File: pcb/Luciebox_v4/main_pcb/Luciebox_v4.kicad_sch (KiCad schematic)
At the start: 67 parts, among them J1 USB_B_Mini, P1 Power, P2 Analog, P3 Digital, P4 Digital, P5 CONN_01X01, P6 CONN_01X01, P7 CONN_01X01, P8 CONN_01X01, Q1 N-Channel_Mosfet, T1 terminal_3x1, T10 terminal_8x1, T11 terminal_8x1, T12 terminal_8x1, T13 terminal_8x1, T2 terminal_3x1, T3 terminal_3x1, T4 terminal_3x1, T5 terminal_8x1, T6 terminal_8x1, T7 terminal_3x1, T8 terminal_3x1, T9 terminal_3x1, U1 CA56-12SRWA, U2 8X8PADS, U3 ATmega328-PU, Y1 16MHz

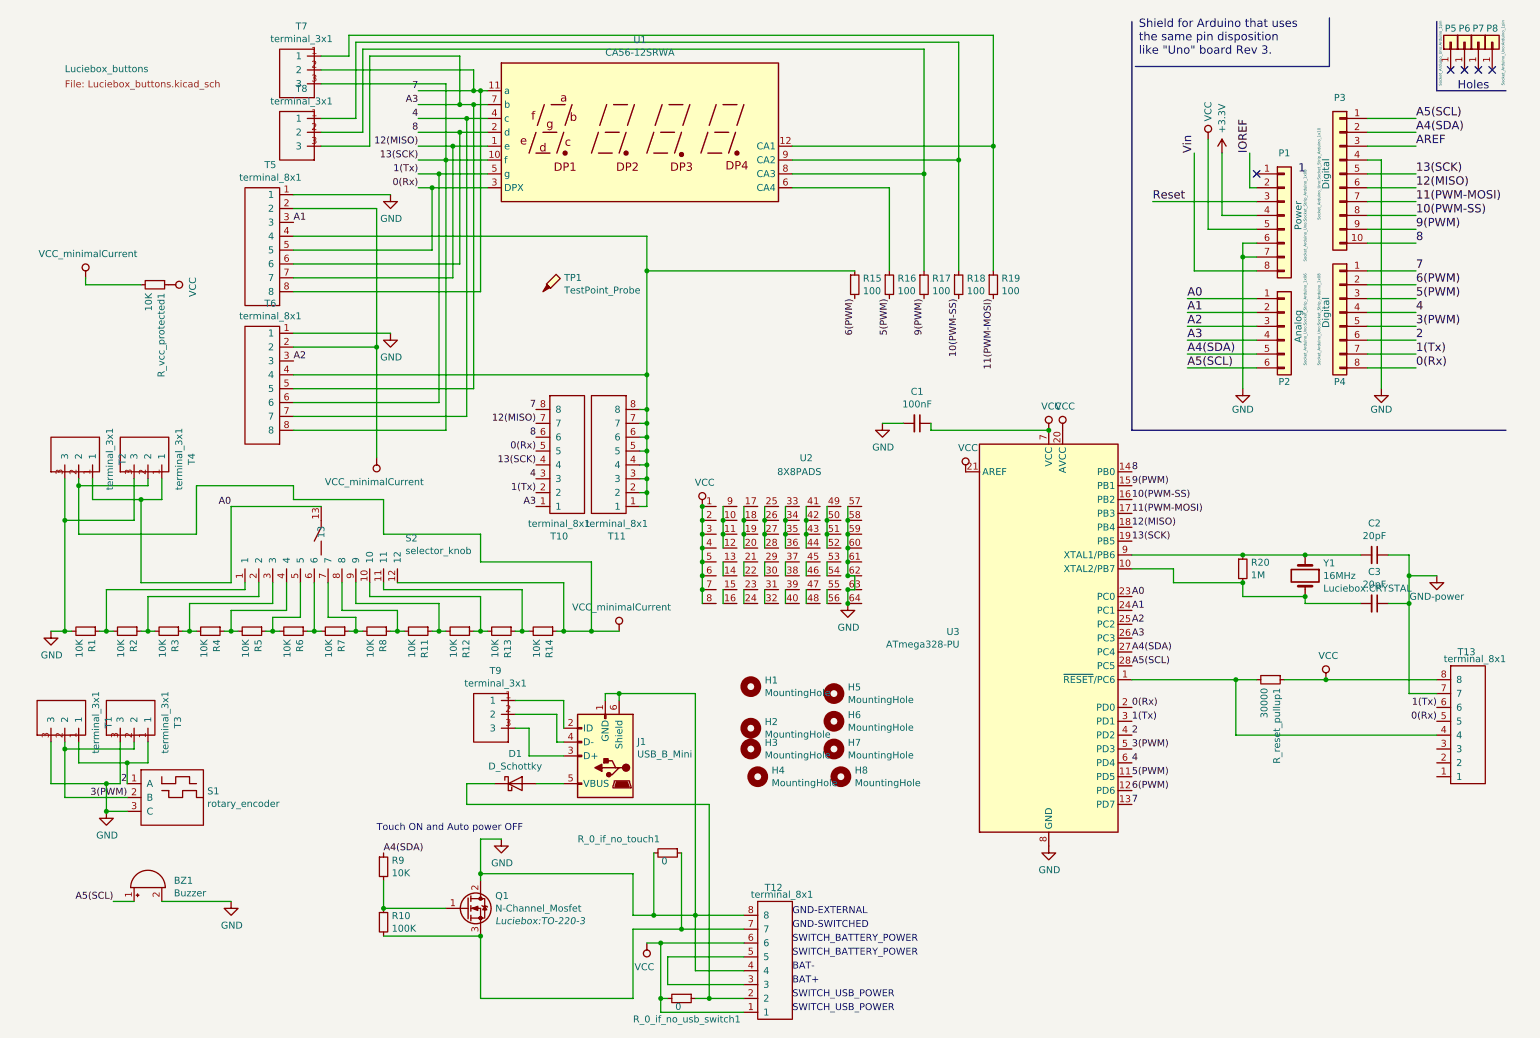
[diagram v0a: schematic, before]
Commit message: V4 main pcb ready for layouting
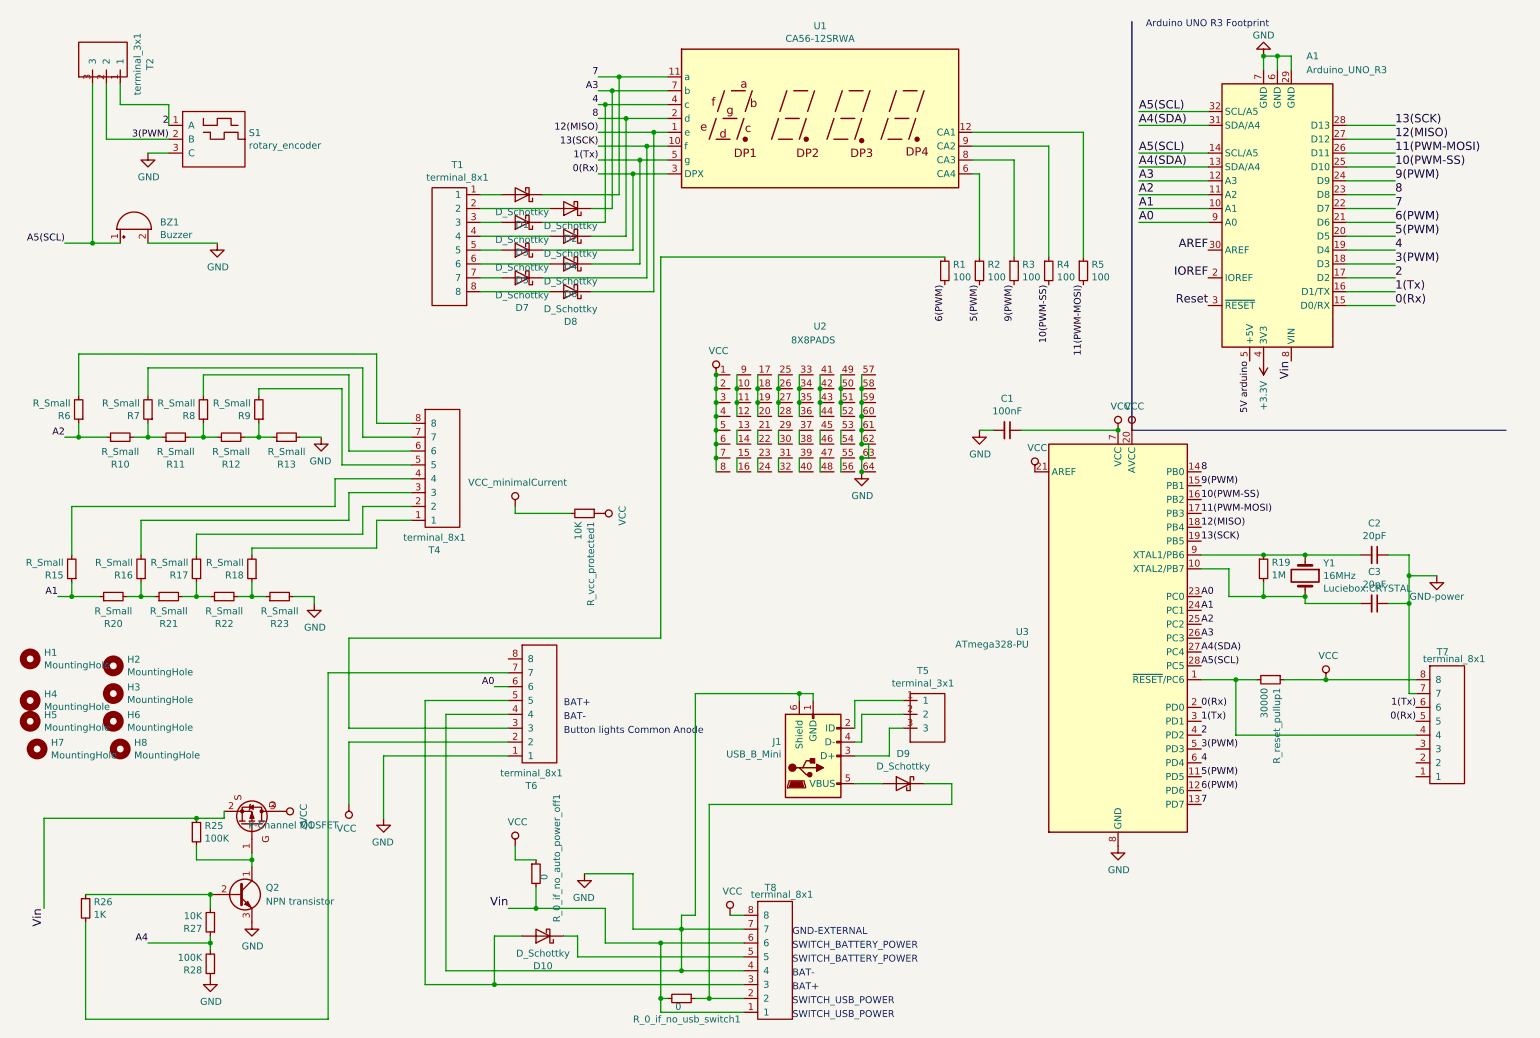
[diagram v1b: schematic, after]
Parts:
- removed P1: Power, Socket_Arduino_Uno:Socket_Strip_Arduino_1x08, symbol Luciebox_components:Conn_01x08-Connector_Generic
- removed P2: Analog, Socket_Arduino_Uno:Socket_Strip_Arduino_1x06, symbol Luciebox_components:Conn_01x06-Connector_Generic
- removed P3: Digital, Socket_Arduino_Uno:Socket_Strip_Arduino_1x10, symbol Luciebox_components:Conn_01x10-Connector_Generic
- removed P4: Digital, Socket_Arduino_Uno:Socket_Strip_Arduino_1x08, symbol Luciebox_components:Conn_01x08-Connector_Generic
- removed P5, P6, P7, P8: CONN_01X01, Socket_Arduino_Uno:Arduino_1pin, symbol Luciebox_components:Conn_01x01-Connector_Generic
- removed Q1: N-Channel_Mosfet, Luciebox:TO-220-3, symbol Luciebox_components:N-Channel_Mosfet
- removed R1, R11, R12, R13, R14, R2, R3, R4, R5, R6, R7, R8, R9: 10K, Luciebox:1206_0805, symbol Luciebox_components:R_Small-Device
- removed R10: 100K, Luciebox:1206_0805, symbol Luciebox_components:R_Small-Device
- removed R_0_if_no_touch1: 0, Luciebox:1206_0805, symbol Luciebox_components:R_Small-Device
- removed S2: selector_knob, Luciebox:Rotary_Switch, symbol Luciebox_components:selector_knob
- removed T10, T11: terminal_8x1, Luciebox:Terminal_8x1_100mil, symbol Luciebox_components:terminal_8x1
- removed T2, T3, T4, T7, T8: terminal_3x1, Luciebox:Terminal_3x1_100mil, symbol Luciebox_components:terminal_3x1
- removed TP1: TestPoint_Probe, symbol Connector:TestPoint_Probe
- added A1: Arduino_UNO_R3, Module:Arduino_UNO_R3, symbol Luciebox_components:Arduino_UNO_R3
- added D1, D10, D2, D3, D4, D5, D6, D7, D8: D_Schottky, Luciebox:D_SMA, symbol Luciebox_components:D_Schottky
- added Q1: P-Channel MOSFET, Package_TO_SOT_SMD:SOT-23, symbol Luciebox_components:P-Channel MOSFET
- added Q2: NPN transistor, Luciebox:SOT-23, symbol Luciebox_components:NPN transistor
- added R10, R11, R12, R13, R15, R16, R17, R18, R20, R21, R22, R23, R6, R7, R8, R9: R_Small, Luciebox:0603_1608Metric, symbol Luciebox_components:R_Small
- added R25, R28: 100K, Luciebox:0603_1608Metric, symbol Luciebox_components:R_Small-Device
- added R26: 1K, Luciebox:0603_1608Metric, symbol Luciebox_components:R_Small-Device
- added R27: 10K, Luciebox:0603_1608Metric, symbol Luciebox_components:R_Small-Device
- added R_0_if_no_auto_power_off1: 0, Luciebox:0603_1608Metric, symbol Luciebox_components:R_Small-Device
- added T6: terminal_8x1, Luciebox:Terminal_8x1_100mil, symbol Luciebox_components:terminal_8x1
- C1, C2, C3: footprint Luciebox:0805 -> Luciebox:0603_1608Metric
- D9: renamed from D1; footprint Luciebox:smd_throughhole_2_pins -> Luciebox:D_SMA
- R1: renamed from R15; footprint Luciebox:1206_0805 -> Luciebox:0603_1608Metric
- R19: renamed from R20; footprint Luciebox:1206_0805 -> Luciebox:0603_1608Metric
- R2: renamed from R16; footprint Luciebox:1206_0805 -> Luciebox:0603_1608Metric
- R3: renamed from R17; footprint Luciebox:1206_0805 -> Luciebox:0603_1608Metric
- R4: renamed from R18; footprint Luciebox:1206_0805 -> Luciebox:0603_1608Metric
- R5: renamed from R19; footprint Luciebox:1206_0805 -> Luciebox:0603_1608Metric
- R_0_if_no_usb_switch1, R_reset_pullup1, R_vcc_protected1: footprint Luciebox:1206_0805 -> Luciebox:0603_1608Metric
- renumbered H5 to H2, H6 to H3, H2 to H4, H3 to H5, H7 to H6, H4 to H7, T5 to T1, T1 to T2, T6 to T4, T9 to T5, T13 to T7, T12 to T8
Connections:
- net +3V3: now also A1.4 (3V3)
- net 0(Rx): now also A1.15 (D0/RX), D5.1 (K); no longer T1.5
- net 1(Tx): now also A1.16 (D1/TX), D6.1 (K); no longer T4.6
- net 10(PWM-SS): now also A1.25 (D10)
- net 11(PWM-MOSI): now also A1.26 (D11)
- net 12(MISO): now also A1.27 (D12), D8.1 (K); no longer T1.7
- net 13(SCK): now also A1.28 (D13), D7.1 (K); no longer T4.8
- net 2: now also A1.17 (D2)
- net 3(PWM): now also A1.18 (D3)
- net 4: now also A1.19 (D4), D3.1 (K); no longer T4.7
- net 5(PWM): now also A1.20 (D5)
- net 6(PWM): now also A1.21 (D6)
- net 7: now also A1.22 (D7), D1.1 (K); no longer T1.8
- net 8: now also A1.23 (D8), D4.1 (K); no longer T1.6
- net 9(PWM): now also A1.24 (D9)
- net A0: now also A1.9 (A0), T6.6
- net A1: now also A1.10 (A1), R15.1, R20.1; no longer T1.3
- net A2: now also A1.11 (A2), R10.1, R6.1; no longer T4.3
- net A3: now also A1.12 (A3), D2.1 (K); no longer T4.5
- net A4(SDA): now also A1.13 (SDA/A4), A1.31 (SDA/A4)
- net A5(SCL): now also T2.3, A1.14 (SCL/A5), A1.32 (SCL/A5)
- net AREF: now also A1.30 (AREF)
- net GND: now also T8.7, A1.29 (GND), A1.6 (GND), A1.7 (GND), Q2.3 (E), R13.2, R23.2, R28.1, T6.1, T6.4; no longer T1.1, T2.3, T4.1, T8.8
- net IOREF: now also A1.2 (IOREF)
- net Reset: now also A1.3 (~{RESET})
- net VCC: now also T8.8, Q1.3 (D), R_0_if_no_auto_power_off1.1, T6.2; no longer R_0_if_no_usb_switch1.2, T8.1, T8.6
- net VCC_minimalCurrent: no longer T1.2, T4.2
- net Vin: now also R_0_if_no_usb_switch1.2, T8.1, T8.6, A1.8 (VIN), Q1.2 (S), R25.1, R_0_if_no_auto_power_off1.2
- net at T8.3: now also D10.2 (A), T6.5; no longer T8.5
- new net: D8.2 (A), T1.8
- new net: Q2.2 (B), R26.1, R27.2
- new net: R26.2, T6.7
- new net: Q1.1 (G), Q2.1 (C), R25.2
- new net: R18.2, T4.1
- new net: R17.2, T4.2
- new net: R16.2, T4.3
- new net: R15.2, T4.4
- new net: R9.2, T4.5
- new net: R8.2, T4.6
- new net: R7.2, T4.7
- new net: R6.2, T4.8
- new net: D6.2 (A), T1.6
- new net: R17.1, R21.2, R22.1
- new net: D1.2 (A), T1.1
- new net: D2.2 (A), T1.2
- new net: D3.2 (A), T1.3
- new net: D4.2 (A), T1.4
- new net: D5.2 (A), T1.5
- new net: D7.2 (A), T1.7
- new net: R12.2, R13.1, R9.1
- new net: R18.1, R22.2, R23.1
- new net: R11.2, R12.1, R8.1
- new net: R16.1, R20.2, R21.1
- new net: R10.2, R11.1, R7.1
- new net: D10.1 (K), T8.5
- new net: R1.1, T6.3
- new net 5V arduino: A1.5 (+5V)
- new net A4: R27.1, R28.2
- no-connect marks 5 -> 0
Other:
- removed sheet Luciebox_buttons
- note added: "Arduino UNO R3 Footprint"
- note added: "Button lights Common Anode"
- note removed: "1"
- note removed: "GND-SWITCHED"
- note removed: "Holes"
- note removed: "Shield for Arduino that uses the same pin disposition like "Uno" board Rev 3."
- note removed: "Touch ON and Auto power OFF"
- moved on the sheet: BZ1, C1, D9, H1, H2, H3, H4, H5, H6, H7, H8, J1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
